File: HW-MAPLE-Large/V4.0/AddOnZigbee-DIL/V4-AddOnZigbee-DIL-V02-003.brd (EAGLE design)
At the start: 33 x 17 mm, 5 parts

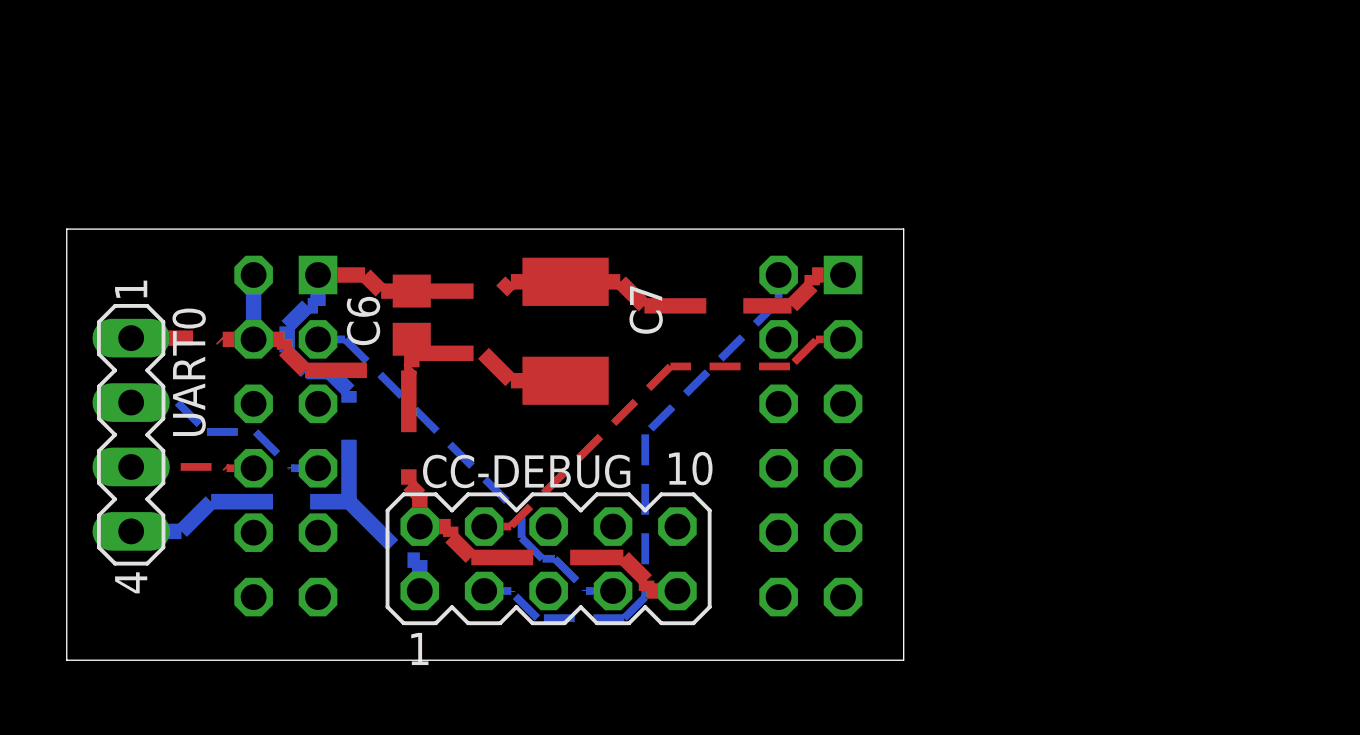
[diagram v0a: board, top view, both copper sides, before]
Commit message: V4-AddOns ; Large
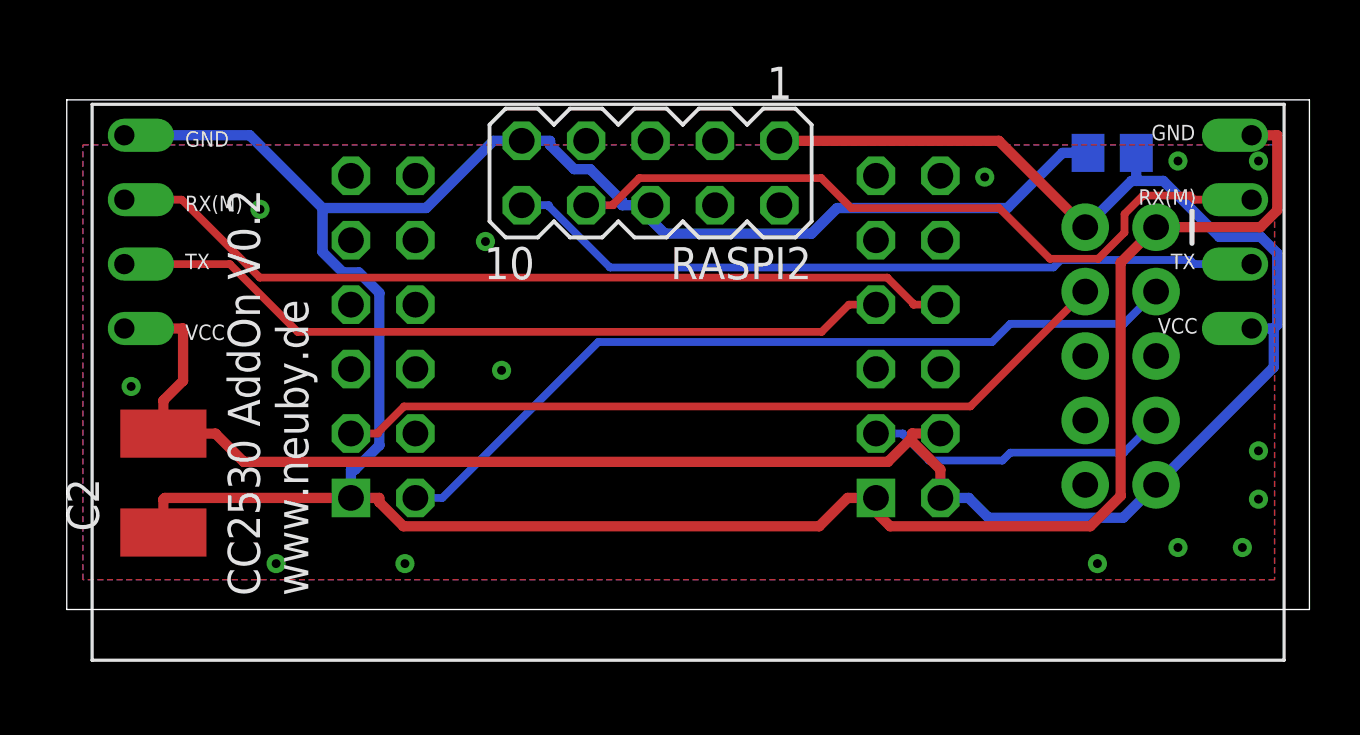
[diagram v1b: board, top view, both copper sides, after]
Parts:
- removed C6: 22pF, rcl:C0805
- removed C7: (no value), rcl:C1812
- removed UART0: (no value), con-lstb:MA04-1
- added C1: 22pF, rcl:C0805
- added C2: (no value), rcl:C1812
- added RASPI2: (no value), con-lstb:MA05-2
- added U$1: MAPLE-CUL-ADDON-V01, Martin-Communication-V4:MAPLE-CUL-V01
- CC-DEBUG: device con-lstb:MA05-2 -> SparkFun-Connectors:2X5-SHROUDED_LOCK
- moved U$3 32.3 mm to (8.89, 21.6), turned to 180 degrees
- moved CC-DEBUG 23.9 mm to (41.6, 12.0), flipped to the bottom
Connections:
- new net RASPI-RX: RASPI2.8, U$1.RX-MAP1
- new net RASPI-TX: RASPI2.10, U$1.TX-MAP1
- net GND: now also C1.2, C2.1, RASPI2.6, RASPI2.9, U$1.GND, U$1.GND1; no longer C6.2, C7.1, UART0.4
- net RX0: now also U$1.RX-MAP; no longer UART0.3
- net TX0: now also U$1.TX-MAP; no longer UART0.2
- net VCC: now also C1.1, C2.2, RASPI2.1, U$1.VCC, U$1.VCC1; no longer C6.1, C7.2, UART0.1
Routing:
- net GND: track 47.5 -> 119.0 mm, vias 0 -> 14
- net VCC: track 40.1 -> 86.7 mm
- net RASPI-TX: track 0.00 -> 30.0 mm
- net RASPI-RX: track 0.00 -> 29.6 mm
- net RX0: track 4.85 -> 33.9 mm
- net TX0: track 8.46 -> 31.2 mm
- net DD: track 17.3 -> 31.3 mm
- net DC: track 22.1 -> 32.6 mm
- net RST: track 16.3 -> 12.2 mm
- added copper zone on layer 1, net GND
- added copper zone on layer 16, net GND
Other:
- board size 33 x 17 mm -> 49 x 20.1 mm
- board text added: "CC2530 AddOn V0.2 www.neuby.de"
